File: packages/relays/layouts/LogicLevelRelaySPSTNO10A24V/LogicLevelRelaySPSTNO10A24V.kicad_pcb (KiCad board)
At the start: 2 copper layers, 6 parts

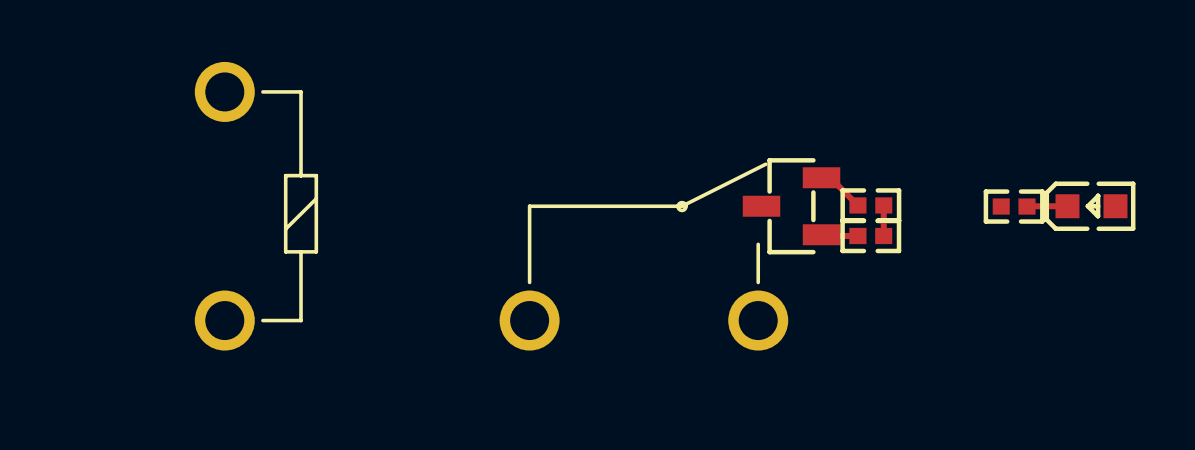
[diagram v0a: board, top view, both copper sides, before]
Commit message: layout
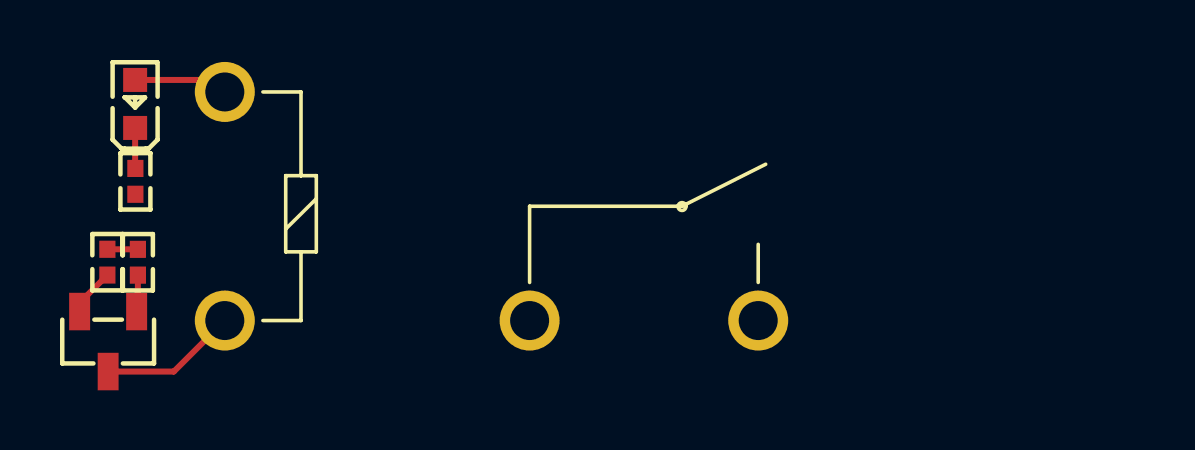
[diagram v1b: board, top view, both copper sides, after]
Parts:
- moved LED1 32.1 mm to (-11.9, -3.41), turned to 90 degrees
- moved R3 29.3 mm to (-11.9, -0.83), turned to -90 degrees
- moved R1 25.5 mm to (-12.8, 1.86), turned to -90 degrees
- moved R2 24.4 mm to (-11.8, 1.87), turned to -90 degrees
- moved Q1 23.2 mm to (-12.8, 4.51), turned to 90 degrees
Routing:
- net contacts[1]: track 0.10 -> 4.69 mm
- net anode: track 0.00 -> 3.16 mm
